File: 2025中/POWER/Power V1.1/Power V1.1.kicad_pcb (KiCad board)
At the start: 2 copper layers, 72.8 x 38.9 mm, 26 parts, among them J1 Conn_01x02_Pin, J2 Conn_01x02_Pin, SW1 SW_SPST, U1 LM2576SX-5.0_NOPB, U2 AZ1117CH-3.3TRG1

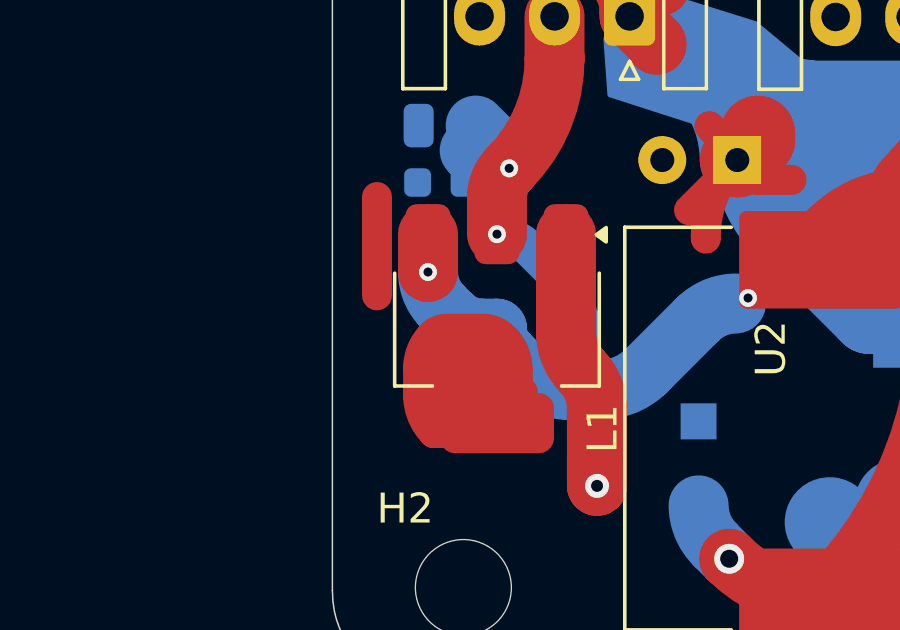
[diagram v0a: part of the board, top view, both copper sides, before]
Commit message: 定期更新
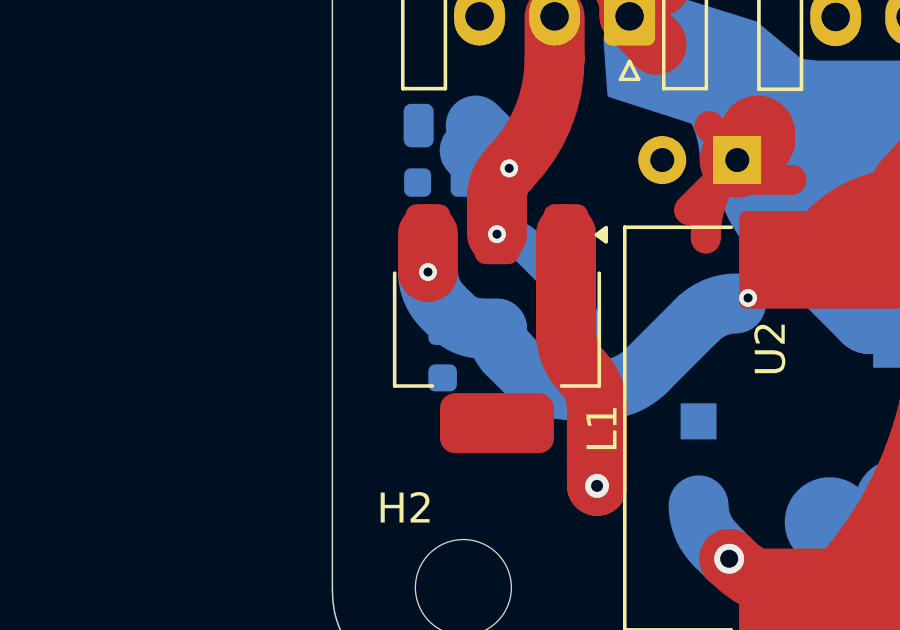
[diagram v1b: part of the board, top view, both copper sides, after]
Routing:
- net unconnected-(U2-EPAD-Pad4): track 20.4 -> 0.00 mm
- net (no net): track 3.28 -> 0.00 mm
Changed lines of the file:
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@@
-	)
-	(segment
-		(start 115.12 170.48)
-		(end 115.12 173.76)
-		(width 1)
-		(layer "F.Cu")
-		(net 0)
 	)
 	(segment
@@
 		(net 9)
 	)
-	(segment
-		(start 116.49 176.188538)
-		(end 116.49 177.090609)
-		(width 1)
-		(layer "F.Cu")
-		(net 10)
-	)
-	(segment
-		(start 117.232 175.641)
-		(end 117.676851 175.641)
-		(width 1)
-		(layer "F.Cu")
-		(net 10)
-	)
-	(segment
-		(start 117.232 176.663464)
-		(end 117.232 175.641)
-		(width 1)
-		(layer "F.Cu")
-		(net 10)
-	)
-	(segment
-		(start 117.01 178.346)
-		(end 118.332966 178.346)
-		(width 1)
-		(layer "F.Cu")
-		(net 10)
-	)
-	(segment
-		(start 117.446 176.424)
-		(end 117.91588 176.424)
-		(width 1)
-		(layer "F.Cu")
-		(net 10)
-	)
-	(segment
-		(start 117.01 178.346)
-		(end 117.01 177.532581)
-		(width 1)
-		(layer "F.Cu")
-		(net 10)
-	)
-	(segment
-		(start 119.078281 178.12072)
-		(end 118.85 178.349)
-		(width 1)
-		(layer "F.Cu")
-		(net 10)
-	)
-	(segment
-		(start 117.446 177.005)
-		(end 117.446 176.424)
-		(width 1)
-		(layer "F.Cu")
-		(net 10)
-	)
-	(segment
-		(start 119.12 178.02)
-		(end 117.54347 178.02)
-		(width 1)
-		(layer "F.Cu")
-		(net 10)
-	)
-	(segment
-		(start 118.662849 174.875)
-		(end 117.440085 174.875)
-		(width 1)
-		(layer "F.Cu")
-		(net 10)
-	)
-	(segment
-		(start 118.694912 175.771911)
-		(end 119.02 176.097)
-		(width 1)
-		(layer "F.Cu")
-		(net 10)
-	)
-	(segment
-		(start 119.806 176.553613)
-		(end 119.806 176.206)
-		(width 1)
-		(layer "F.Cu")
-		(net 10)
-	)
-	(segment
-		(start 119.201 176.896)
-		(end 117.709149 176.896)
-		(width 1)
-		(layer "F.Cu")
-		(net 10)
-	)
-	(segment
-		(start 119.201 176.533973)
-		(end 119.201 176.896)
-		(width 1)
-		(layer "F.Cu")
-		(net 10)
-	)
-	(segment
-		(start 119.395171 175.214171)
-		(end 119.334 175.153)
-		(width 1)
-		(layer "F.Cu")
-		(net 10)
-	)
-	(arc
-		(start 119.806 176.206)
-		(mid 119.699229 175.669226)
-		(end 119.395171 175.214171)
-		(width 1)
-		(layer "F.Cu")
-		(net 10)
-	)
-	(arc
-		(start 117.676851 175.641)
-		(mid 117.819266 175.612671)
-		(end 117.94 175.532)
-		(width 1)
-		(layer "F.Cu")
-		(net 10)
-	)
-	(arc
-		(start 116.49 177.090609)
-		(mid 116.625144 177.770021)
-		(end 117.01 178.346)
-		(width 1)
-		(layer "F.Cu")
-		(net 10)
-	)
-	(arc
-		(start 119.02 176.097)
-		(mid 119.153959 176.297485)
-		(end 119.201 176.533973)
-		(width 1)
-		(layer "F.Cu")
-		(net 10)
-	)
-	(arc
-		(start 118.332966 178.346)
-		(mid 118.758906 178.261275)
-		(end 119.12 178.02)
-		(width 1)
-		(layer "F.Cu")
-		(net 10)
-	)
-	(arc
-		(start 117.440085 174.875)
-		(mid 117.174853 174.927758)
-		(end 116.95 175.078)
-		(width 1)
-		(layer "F.Cu")
-		(net 10)
-	)
-	(arc
-		(start 119.334 175.153)
-		(mid 119.026073 174.94725)
-		(end 118.662849 174.875)
-		(width 1)
-		(layer "F.Cu")
-		(net 10)
-	)
-	(arc
-		(start 116.95 175.078)
-		(mid 116.60955 175.587519)
-		(end 116.49 176.188538)
-		(width 1)
-		(layer "F.Cu")
-		(net 10)
-	)
-	(arc
-		(start 117.91588 176.424)
-		(mid 118.073975 176.392553)
-		(end 118.208 176.303)
-		(width 1)
-		(layer "F.Cu")
-		(net 10)
-	)
-	(arc
-		(start 119.988 176.993)
-		(mid 119.8533 176.791408)
-		(end 119.806 176.553613)
-		(width 1)
-		(layer "F.Cu")
-		(net 10)
-	)
-	(arc
-		(start 117.709149 176.896)
-		(mid 117.566734 176.924328)
-		(end 117.446 177.005)
-		(width 1)
-		(layer "F.Cu")
-		(net 10)
-	)
-	(arc
-		(start 116.941 177.366)
-		(mid 117.156372 177.043674)
-		(end 117.232 176.663464)
-		(width 1)
-		(layer "F.Cu")
-		(net 10)
-	)
-	(arc
-		(start 118.644 175.649)
-		(mid 118.657231 175.715519)
-		(end 118.694912 175.771911)
-		(width 1)
-		(layer "F.Cu")
-		(net 10)
-	)
-	(arc
-		(start 119.12 178.02)
-		(mid 119.109157 178.074509)
-		(end 119.078281 178.12072)
-		(width 1)
-		(layer "F.Cu")
-		(net 10)
-	)
-	(arc
-		(start 117.01 177.532581)
-		(mid 116.992068 177.442428)
-		(end 116.941 177.366)
-		(width 1)
-		(layer "F.Cu")
-		(net 10)
-	)
 	(zone
